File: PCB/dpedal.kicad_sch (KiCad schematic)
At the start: 26 parts, among them J1 USB_C_Receptacle_USB2.0, J2 Conn_02x10_Counter_Clockwise, J3 Conn_ARM_JTAG_SWD_10, J4 Conn_01x05, SW1 SW_Push, SW10 SW_Push, SW2 SW_Push, SW3 SW_Push, SW4 SW_Push, SW5 RESET, SW6 FLASH, SW7 SW_Push, SW8 SW_Push, SW9 SW_Push, U1 STM32F072C8Tx, U2 LDO

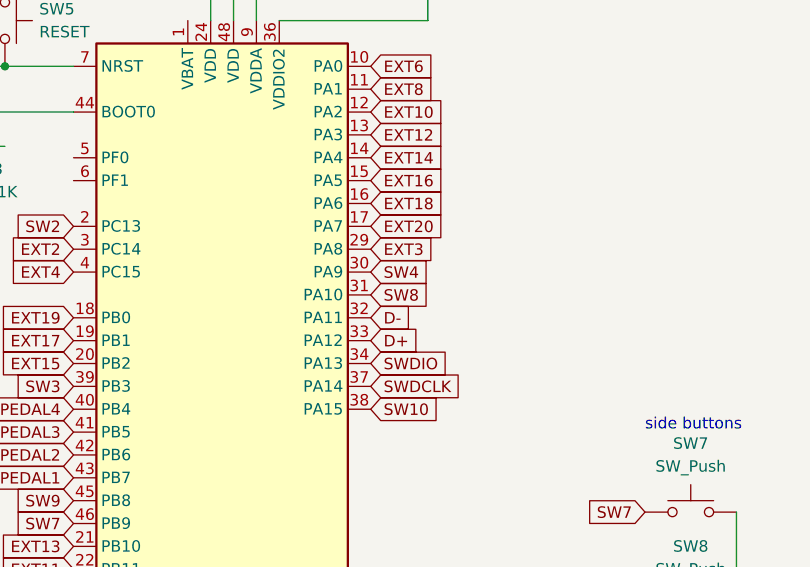
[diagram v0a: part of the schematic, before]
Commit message: Finalize PCB BOM
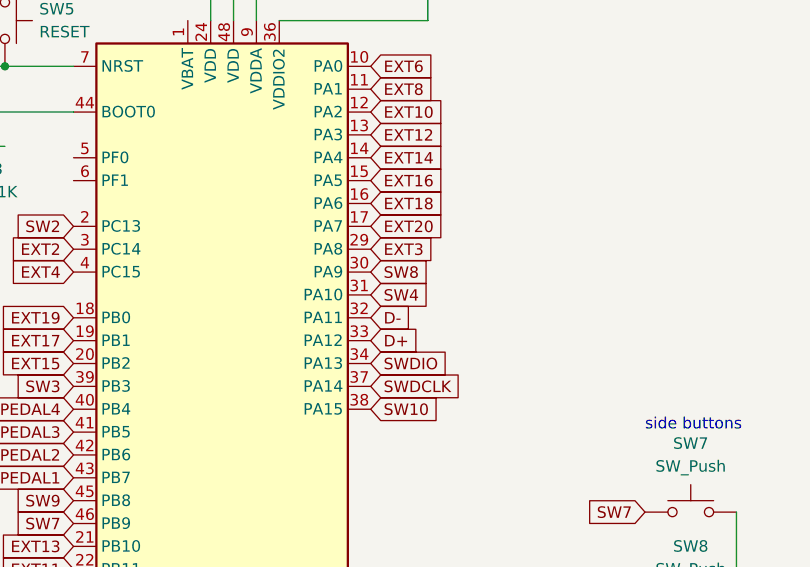
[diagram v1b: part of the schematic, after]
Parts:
- J2: JLCPCB Part # (none) -> C132444
- J4: JLCPCB Part # (none) -> C124405
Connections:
- net SW4: now also U1.31 (PA10); no longer U1.30 (PA9)
- net SW8: now also U1.30 (PA9); no longer U1.31 (PA10)
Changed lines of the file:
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@@
     )
   )
-  (global_label "SW8" (shape input) (at 147.32 90.17 0) (fields_autoplaced)
-    (effects (font (size 1.27 1.27)) (justify left))
-    (property "Intersheetrefs" "${INTERSHEET_REFS}" (at 153.6036 90.2494 0)
+  (global_label "SW4" (shape input) (at 147.32 90.17 0) (fields_autoplaced)
+    (effects (font (size 1.27 1.27)) (justify left))
+    (property "Intersheetrefs" "${INTERSHEET_REFS}" (at 154.0962 90.17 0)
       (effects (font (size 1.27 1.27)) (justify left) hide)
     )
@@
     )
   )
-  (global_label "SW4" (shape input) (at 147.32 87.63 0) (fields_autoplaced)
-    (effects (font (size 1.27 1.27)) (justify left))
-    (property "Intersheetrefs" "${INTERSHEET_REFS}" (at 153.6036 87.7094 0)
+  (global_label "SW8" (shape input) (at 147.32 87.63 0) (fields_autoplaced)
+    (effects (font (size 1.27 1.27)) (justify left))
+    (property "Intersheetrefs" "${INTERSHEET_REFS}" (at 154.0962 87.63 0)
       (effects (font (size 1.27 1.27)) (justify left) hide)
     )
@@
     )
     (property "Datasheet" "~" (at 83.82 102.87 0)
+      (effects (font (size 1.27 1.27)) hide)
+    )
+    (property "JLCPCB Part #" "C132444" (at 83.82 102.87 0)
       (effects (font (size 1.27 1.27)) hide)
     )
@@
       (effects (font (size 1.27 1.27)) hide)
     )
+    (property "JLCPCB Part #" "C124405" (at 82.55 137.16 0)
+      (effects (font (size 1.27 1.27)) hide)
+    )
